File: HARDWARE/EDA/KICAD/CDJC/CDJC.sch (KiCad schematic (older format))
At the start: 63 parts, among them J1 COM_IN, J2 COM_OUT, J3 POWER_IN, J4 POWER_OUT, J5 BIT_OUT, Q1 BC549, SW1 B-SET, U1 74LS04, U2 74LS32, U3 74LS08, U4 74LS08, U5 74LS08, U6 74LS08, U7 74LS32, U8 74LS32, U9 4017

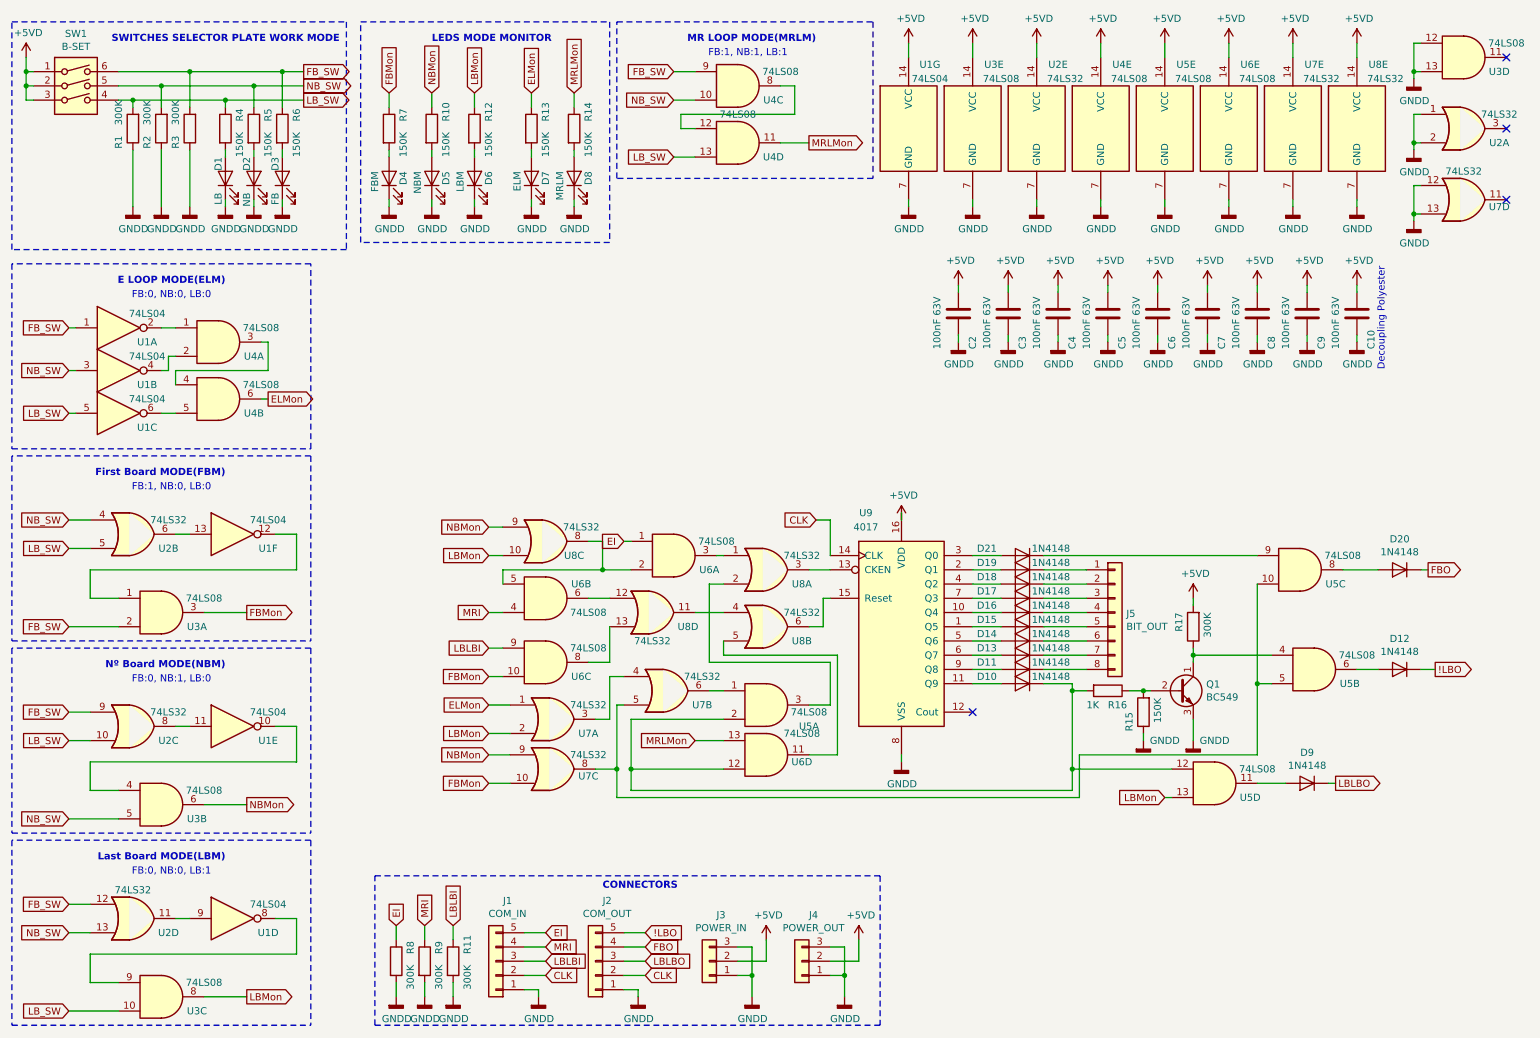
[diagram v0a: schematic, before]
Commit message: pause work for sleep
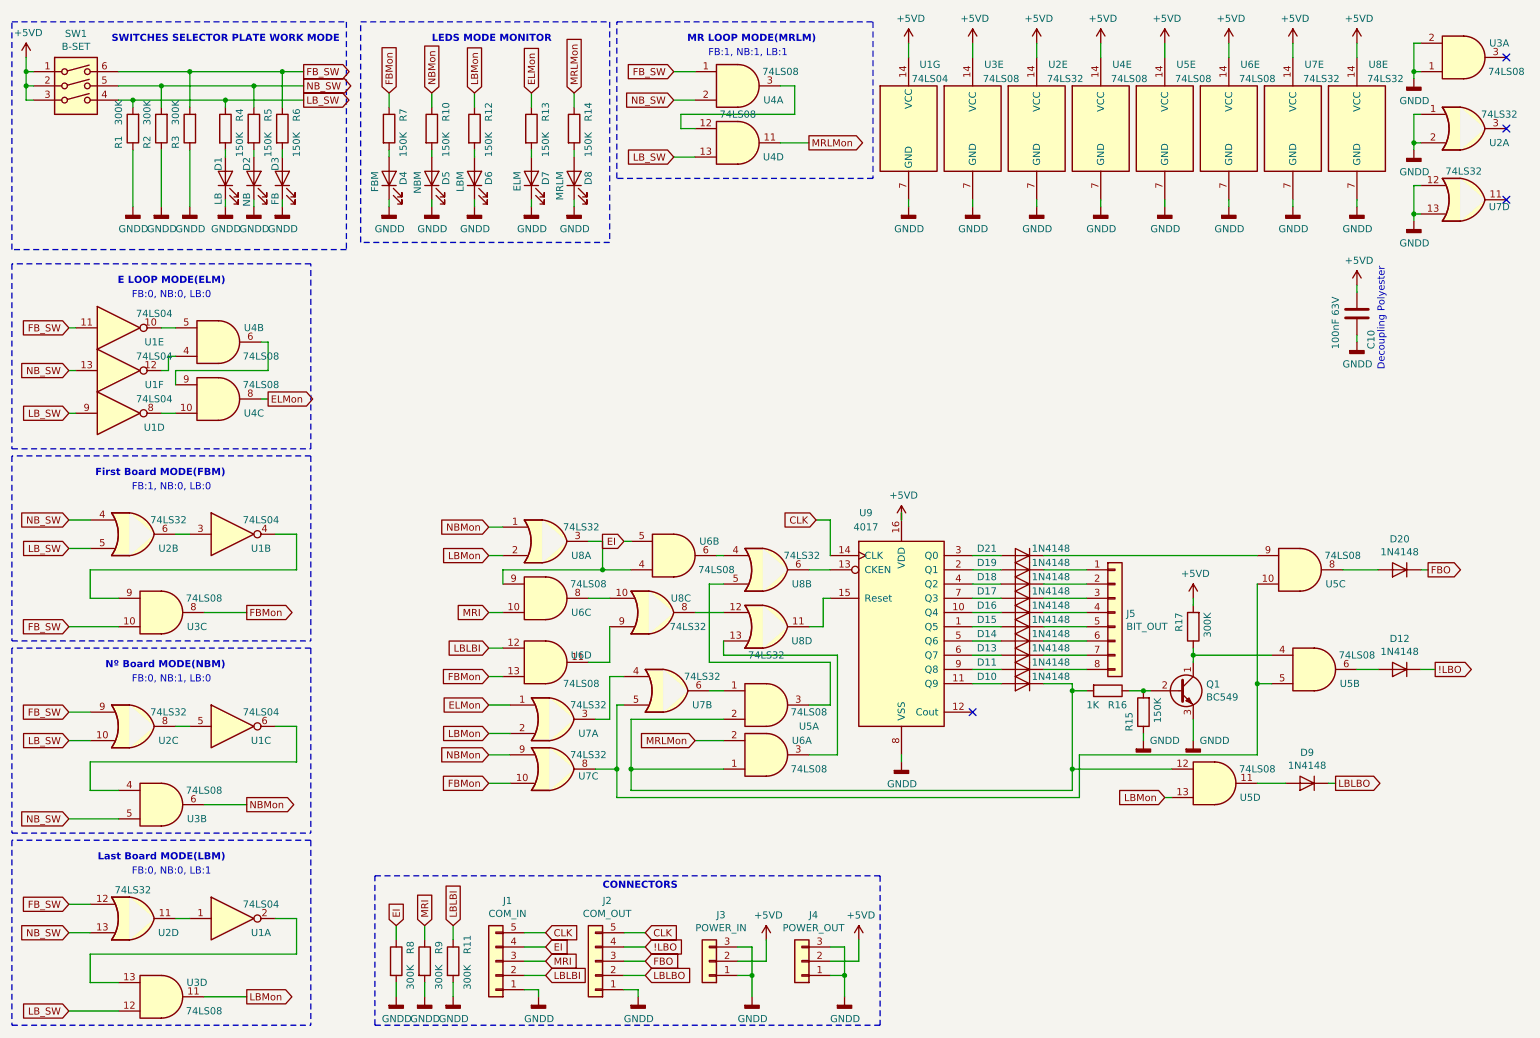
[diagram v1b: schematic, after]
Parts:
- removed C2, C3, C4, C5, C6, C7, C8, C9: 100nF 63V, Capacitor_THT:C_Rect_L7.0mm_W2.5mm_P5.00mm, symbol Device:C
- R11, R8, R9: footprint Resistor_THT:R_Axial_DIN0207_L6.3mm_D2.5mm_P2.54mm_Vertical -> Resistor_THT:R_Axial_DIN0207_L6.3mm_D2.5mm_P7.62mm_Horizontal
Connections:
- net !LBO: now also J2.4 (Pin_4); no longer J2.5 (Pin_5)
- net CLK: now also J1.5 (Pin_5), J2.5 (Pin_5); no longer J1.2 (Pin_2), J2.2 (Pin_2)
- net EI: now also J1.4 (Pin_4), U6.5; no longer J1.5 (Pin_5), U6.1
- net ELMon: now also U4.8; no longer U4.6
- net FBMon: now also U3.8, U6.13; no longer U3.3, U6.10
- net FBO: now also J2.3 (Pin_3); no longer J2.4 (Pin_4)
- net FB_SW: now also U1.11, U3.10, U4.1; no longer U1.1, U3.2, U4.9
- net GNDD: now also U3.1, U3.2; no longer U3.12, U3.13
- net LBLBI: now also J1.2 (Pin_2), U6.12; no longer J1.3 (Pin_3), U6.9
- net LBLBO: now also J2.2 (Pin_2); no longer J2.3 (Pin_3)
- net LBMon: now also U3.11, U8.2; no longer U3.8, U8.10
- net LB_SW: now also U1.9, U3.12; no longer U1.5, U3.10
- net MRI: now also J1.3 (Pin_3), U6.10; no longer J1.4 (Pin_4), U6.4
- net MRLMon: now also U6.2; no longer U6.13
- net NBMon: now also U8.1; no longer U8.9
- net NB_SW: now also U1.13, U4.2; no longer U1.3, U4.10
- net at U4.12: now also U4.3; no longer U4.8
- net at U2.6: now also U1.3; no longer U1.13
- net at U1.10: now also U4.5; no longer U3.4
- net at U2.8: now also U1.5; no longer U1.11
- net at U1.12: now also U4.4; no longer U3.1
- net at U1.8: now also U4.10; no longer U3.9
- net at U1.2: now also U3.13; no longer U4.1
- net at U1.4: now also U3.9; no longer U4.2
- net at U1.6: now also U3.4; no longer U4.5
- net at U2.11: now also U1.1; no longer U1.9
- net at U9.13 (CKEN): now also U8.6; no longer U8.3
- net at U9.15 (Reset): now also U8.11; no longer U8.6
- net at D10.1 (K), R16.2, U5.12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: now also U6.1; no longer U6.12
- net at U8.12: now also U8.8; no longer U6.6
- net at U5.3: now also U8.5; no longer U8.2
- net at U6.3: now also U8.13; no longer U8.1
- net at U8.4: now also U6.6; no longer U8.11
- net at U6.11: now also U8.9; no longer U8.5
- net at U6.8: now also U8.10; no longer U8.13
- new net: U4.6, U4.9
- new net: U6.4, U6.9, U8.3
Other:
- moved on the sheet: U1A, U1B, U1C, U1D, U1E, U1F, U3A, U3C, U3D, U4A, U4B, U4C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
